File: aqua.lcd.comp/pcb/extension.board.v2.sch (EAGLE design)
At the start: 60 parts, among them IC1 NCP1117ST50T3G, T1 IRFR024NPBF, T10 BC847BSMD, T11 IRFR024NPBF, T12 BC847BSMD, T13 BC847BSMD, T2 BC847BSMD, T3 IRFR024NPBF, T4 BC847BSMD, T5 IRFR024NPBF, T6 BC847BSMD, T7 IRFR024NPBF, T8 BC847BSMD, T9 IRFR024NPBF

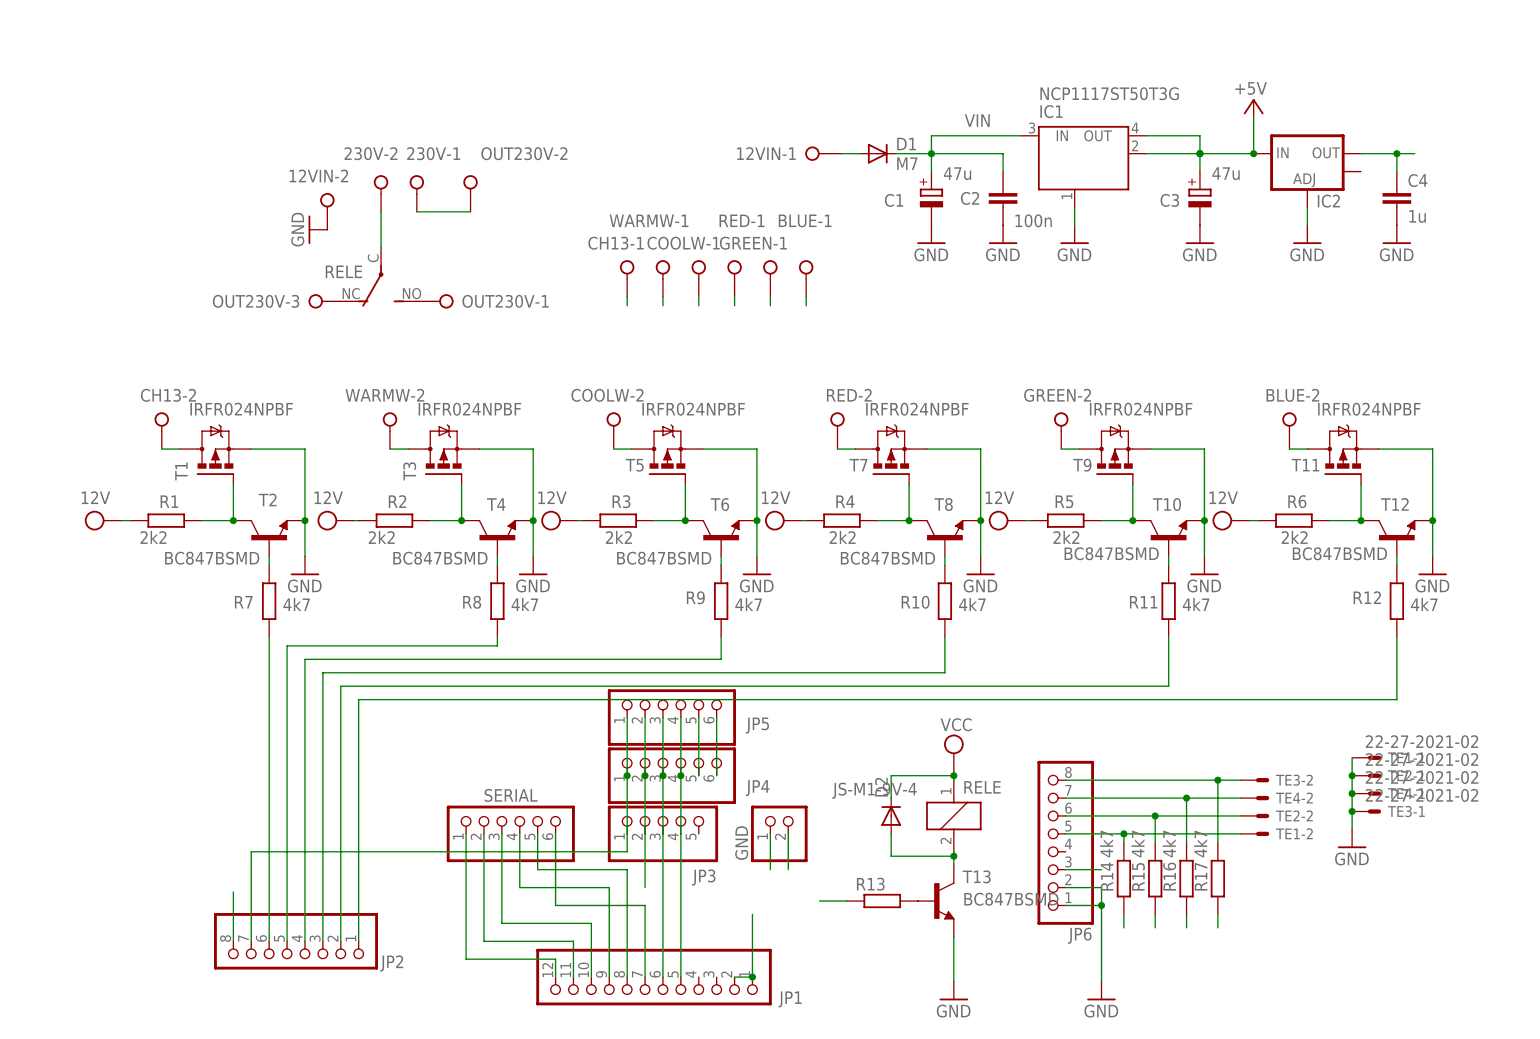
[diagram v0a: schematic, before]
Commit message: first
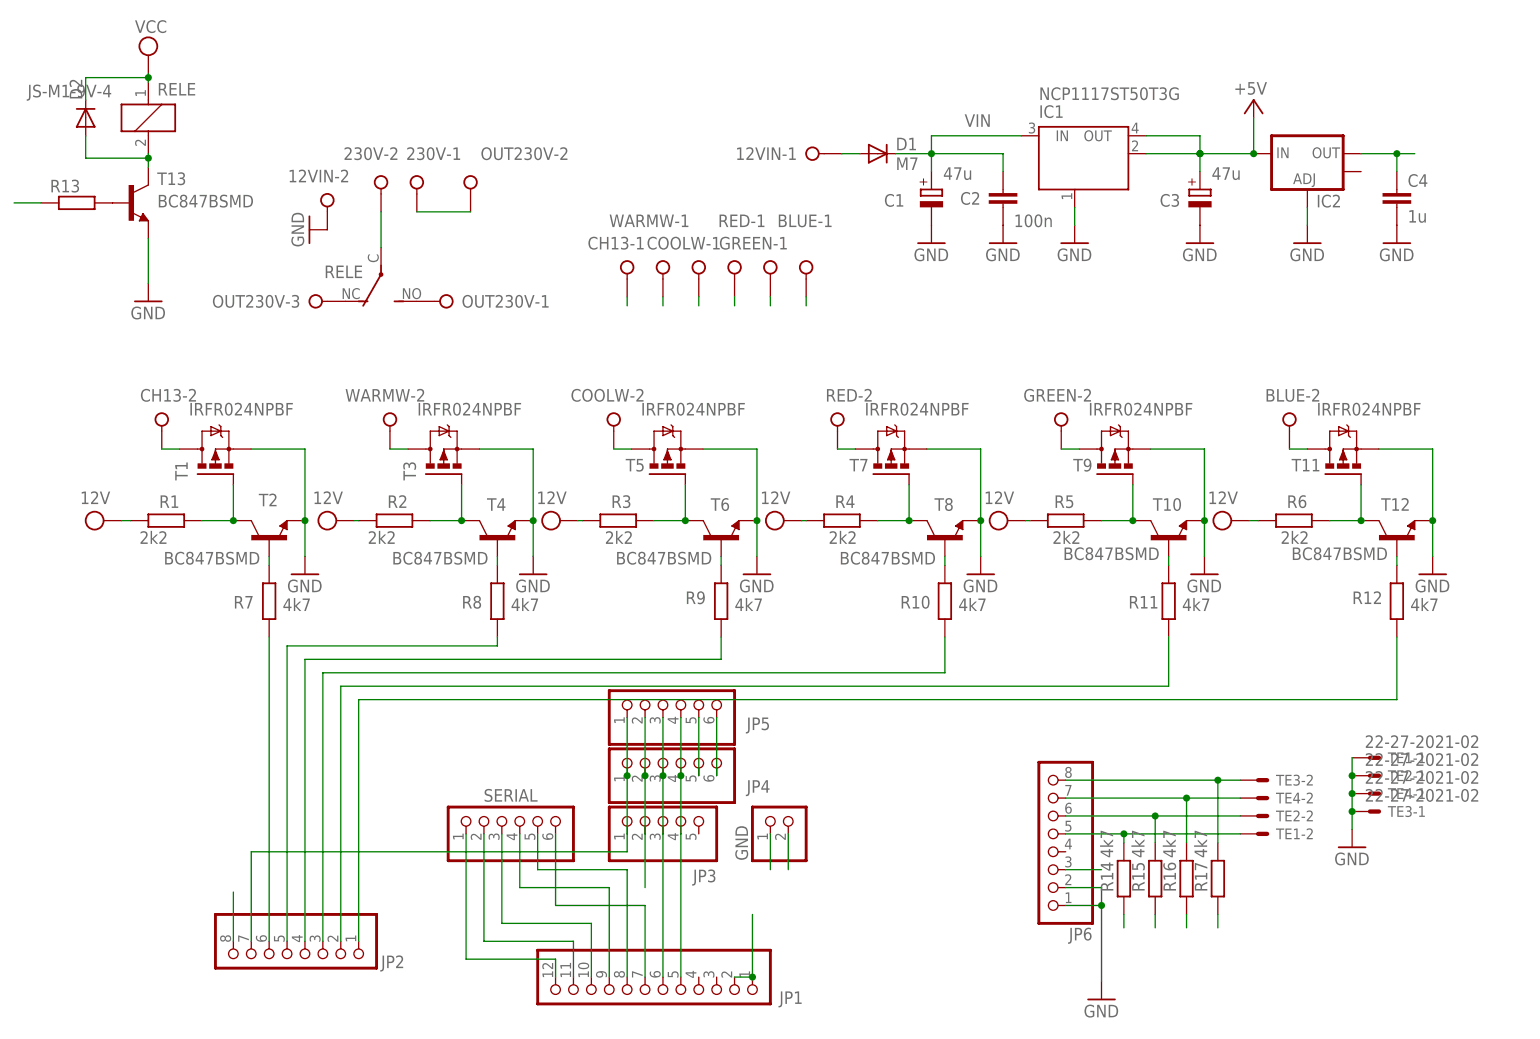
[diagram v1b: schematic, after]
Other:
- moved on the sheet: D2, R13, RELE, T13
